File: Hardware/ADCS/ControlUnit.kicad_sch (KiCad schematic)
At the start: 19 parts, among them SW1 SW_SPDT, U1 STM32L471VET6, Y1 32MHz

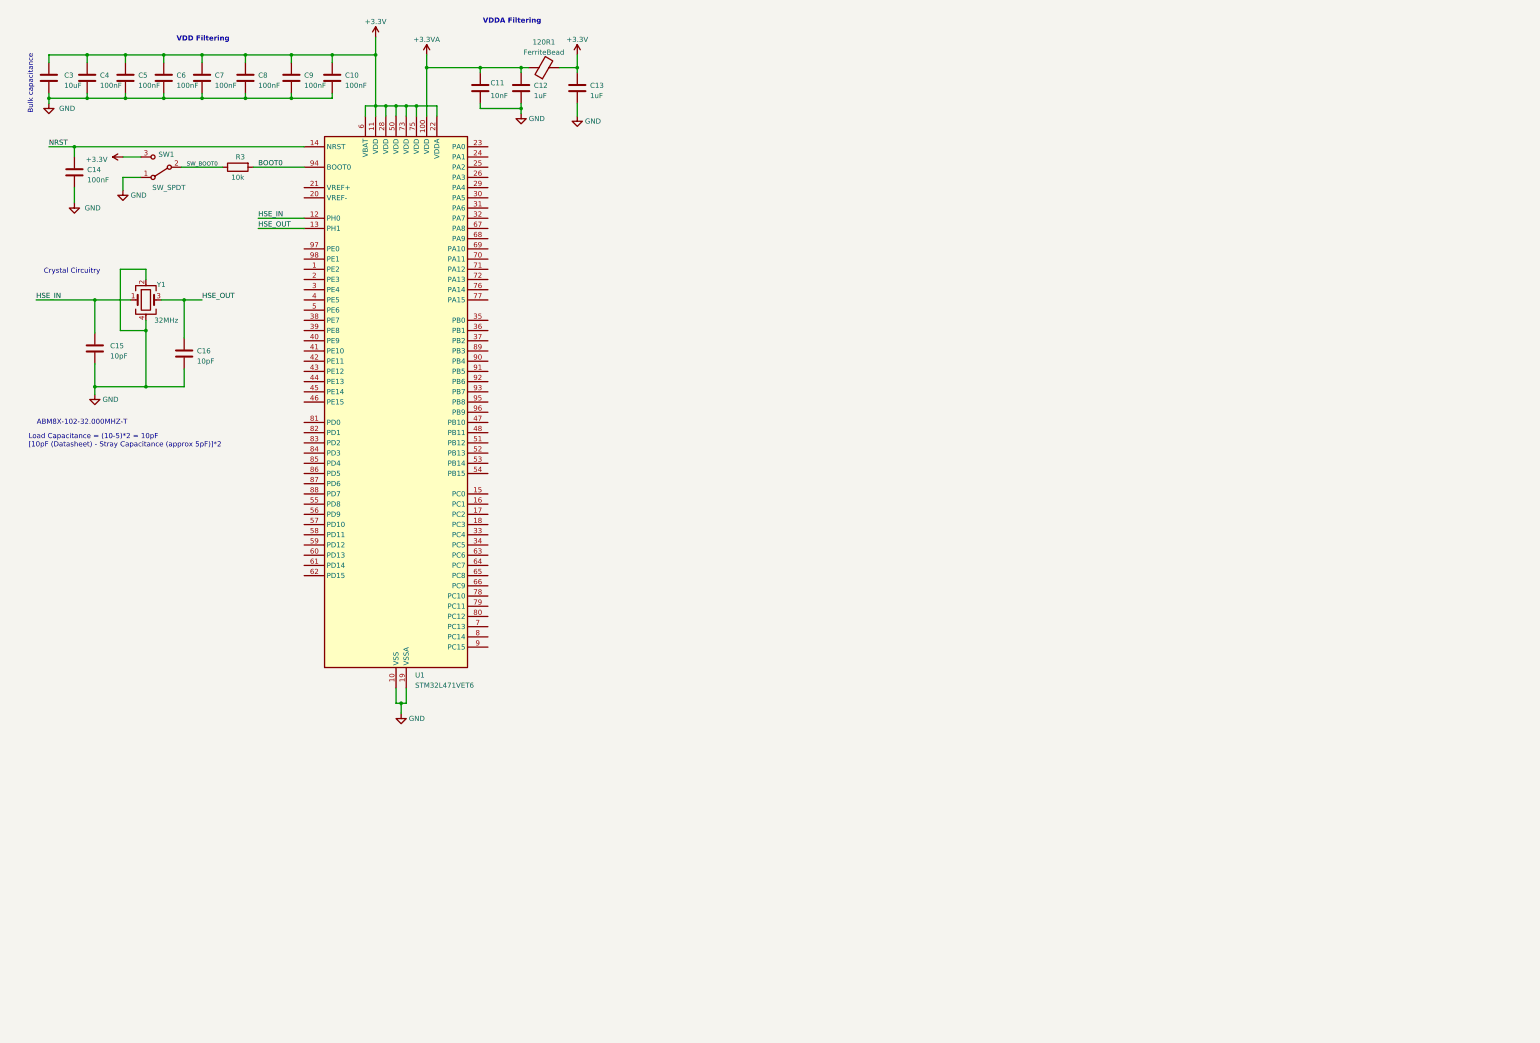
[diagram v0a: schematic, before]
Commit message: ADCS PCB Schematic
Progress in Schematic
Added STM32 Project
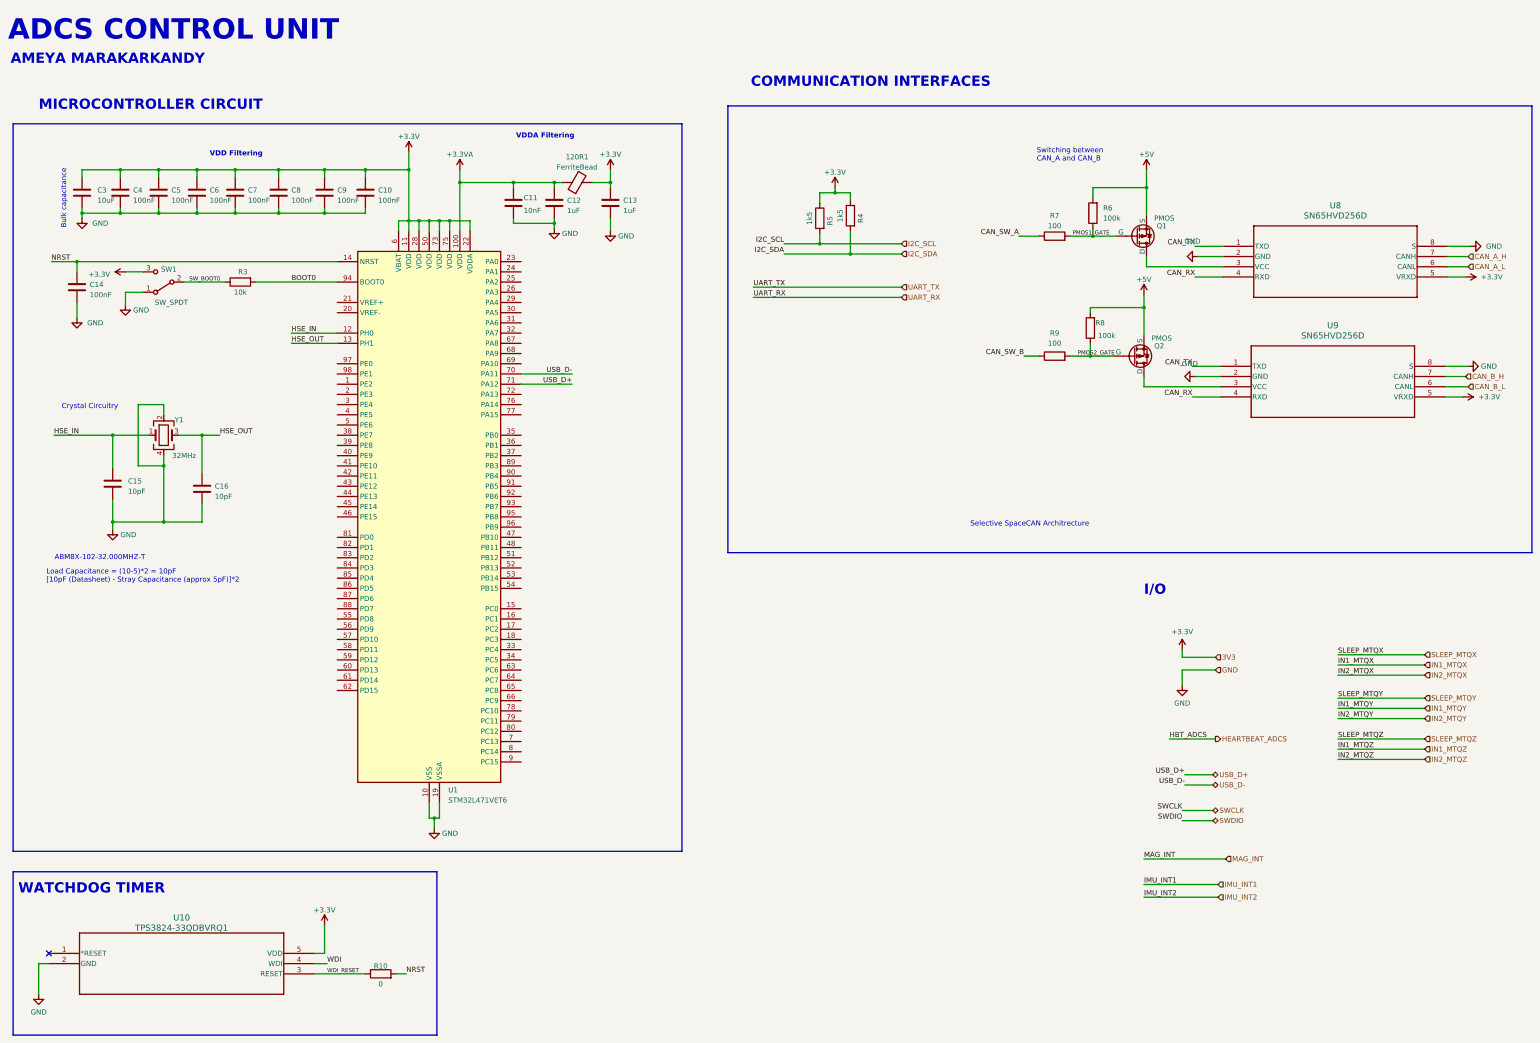
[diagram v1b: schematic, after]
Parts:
- added Q1, Q2: PMOS, Package_TO_SOT_SMD:SOT-23-3, symbol Simulation_SPICE:PMOS
- added R10: 0, Resistor_SMD:R_0603_1608Metric, symbol Device:R
- added R4, R5: 1k5, Resistor_SMD:R_0603_1608Metric, symbol Device:R
- added R6, R8: 100k, Resistor_SMD:R_0603_1608Metric, symbol Device:R
- added R7, R9: 100, Resistor_SMD:R_0603_1608Metric, symbol Device:R
- added U10: TPS3824-33QDBVRQ1, TPS3824:tps3824, symbol TPS3824:TPS3824-33QDBVRQ1
- added U8, U9: SN65HVD256D, SN65HVD:D8, symbol SN65HVD256D:SN65HVD256D
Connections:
- net +3.3V: now also R4.1, R5.1, U10.5 (VDD), U8.5 (VRXD), U9.5 (VRXD)
- net GND: now also U10.2 (GND), U8.2 (GND), U8.8 (S), U9.2 (GND), U9.8 (S)
- net NRST: now also R10.2
- net USB_D-: now reaches U1.70 (PA11)
- net USB_D+: now reaches U1.71 (PA12)
- new net: Q2.1 (D), U9.3 (VCC)
- new net: Q1.1 (D), U8.3 (VCC)
- new net +5V: Q1.3 (S), Q2.3 (S), R6.2, R8.2
- new net CAN_A_H: U8.7 (CANH)
- new net CAN_A_L: U8.6 (CANL)
- new net CAN_B_H: U9.7 (CANH)
- new net CAN_B_L: U9.6 (CANL)
- new net CAN_RX: U8.4 (RXD), U9.4 (RXD)
- new net CAN_SW_A: R7.1
- new net CAN_SW_B: R9.1
- new net CAN_TX: U8.1 (TXD), U9.1 (TXD)
- new net I2C_SCL: R5.2
- new net I2C_SDA: R4.2
- new net PMOS1_GATE: Q1.2 (G), R6.1, R7.2
- new net PMOS2_GATE: Q2.2 (G), R8.1, R9.2
- new net WDI: U10.4 (WDI)
- new net WDI_RESET: R10.1, U10.3 (RESET)
- no-connect marks 0 -> 1
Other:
- note added: "ADCS CONTROL UNIT"
- note added: "AMEYA MARAKARKANDY"
- note added: "COMMUNICATION INTERFACES"
- note added: "I/O"
- note added: "MICROCONTROLLER CIRCUIT"
- note added: "Selective SpaceCAN Architrecture"
- note added: "Switching between CAN_A and CAN_B"
- note added: "WATCHDOG TIMER"
- moved on the sheet: 120R1, C10, C11, C12, C13, C14, C15, C16, C3, C4, C5, C6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

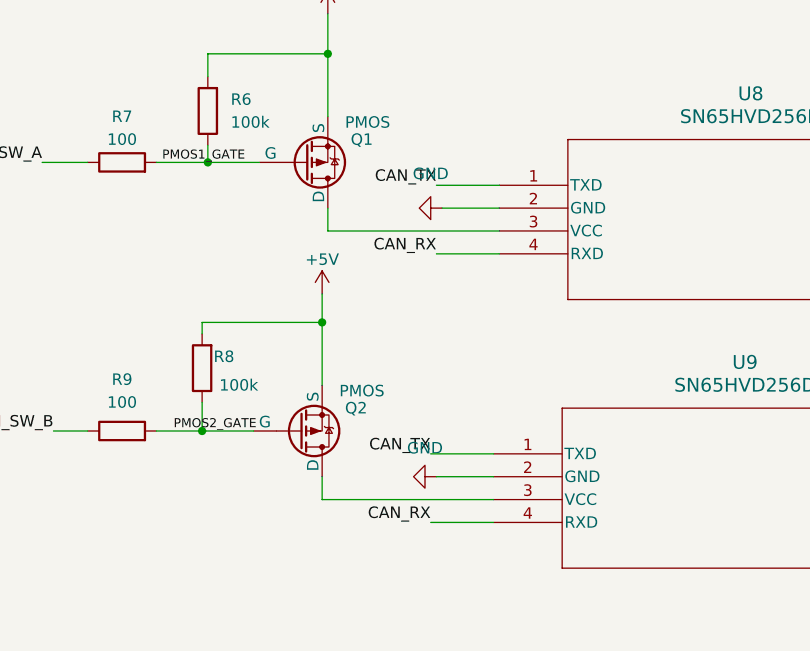
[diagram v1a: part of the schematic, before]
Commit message: ADCS PCB Rough Layout
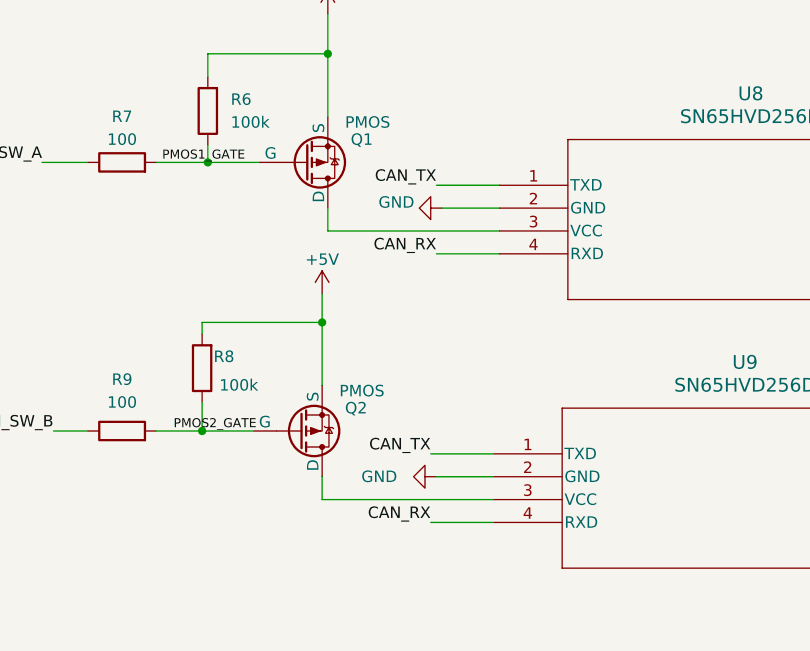
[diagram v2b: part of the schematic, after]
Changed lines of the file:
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@@
 		(on_board yes)
 		(dnp no)
-		(fields_autoplaced yes)
 		(property "Reference" "#PWR055"
 			(at 308.61 107.95 0)
@@
 		)
 		(property "Value" "GND"
-			(at 313.69 104.775 90)
+			(at 308.61 107.95 90)
 			(effects
 				(font
@@
 		(on_board yes)
 		(dnp no)
-		(fields_autoplaced yes)
 		(property "Reference" "#PWR051"
 			(at 309.245 78.105 0)
@@
 		)
 		(property "Value" "GND"
-			(at 314.325 74.295 90)
-			(effects
-				(font
+			(at 310.515 77.47 90)
+			(effects
+				(font
